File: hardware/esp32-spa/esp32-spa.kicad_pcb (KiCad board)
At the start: 2 copper layers, 17 parts, among them J1 RJ45, J2 RJ45, U1 ESP32-DevKitC-32E, U2 PC817, U3 PC817, U4 PC817, U5 PC817

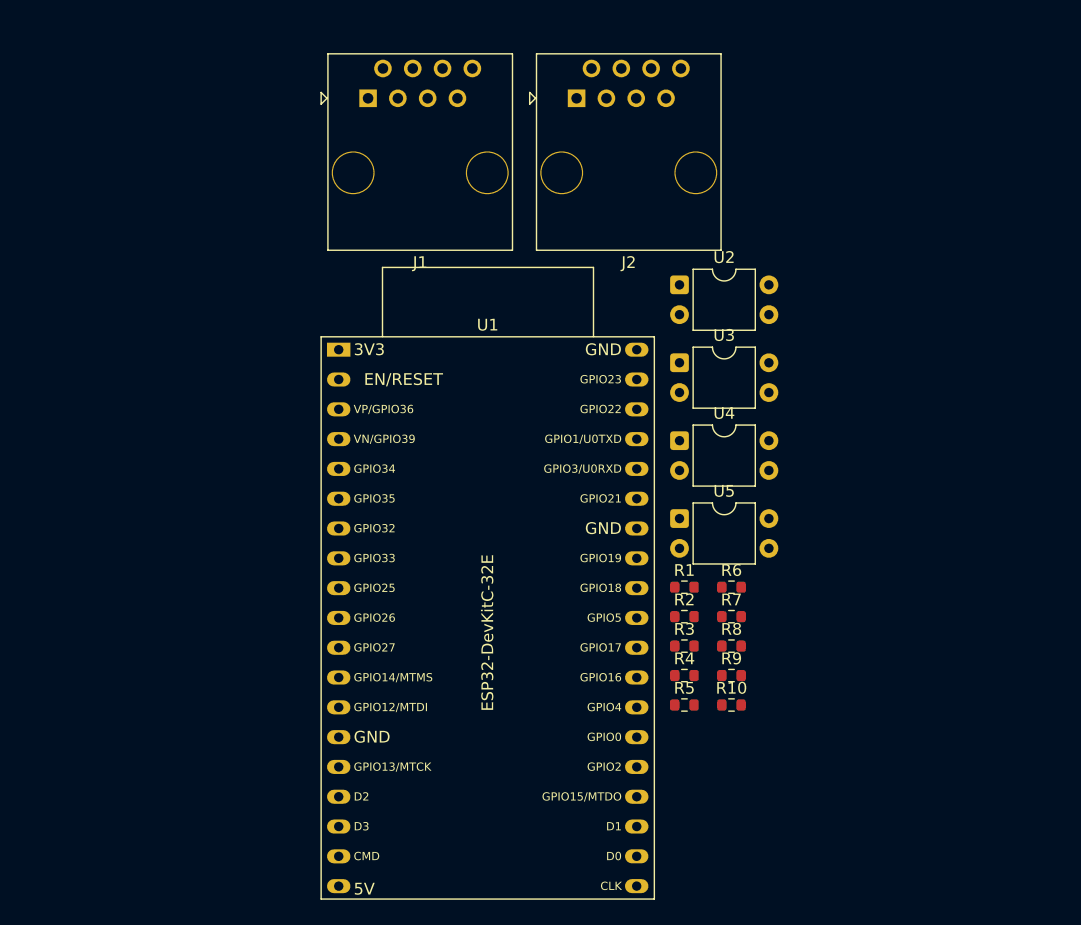
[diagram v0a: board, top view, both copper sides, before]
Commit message: Reorganized pcb layout
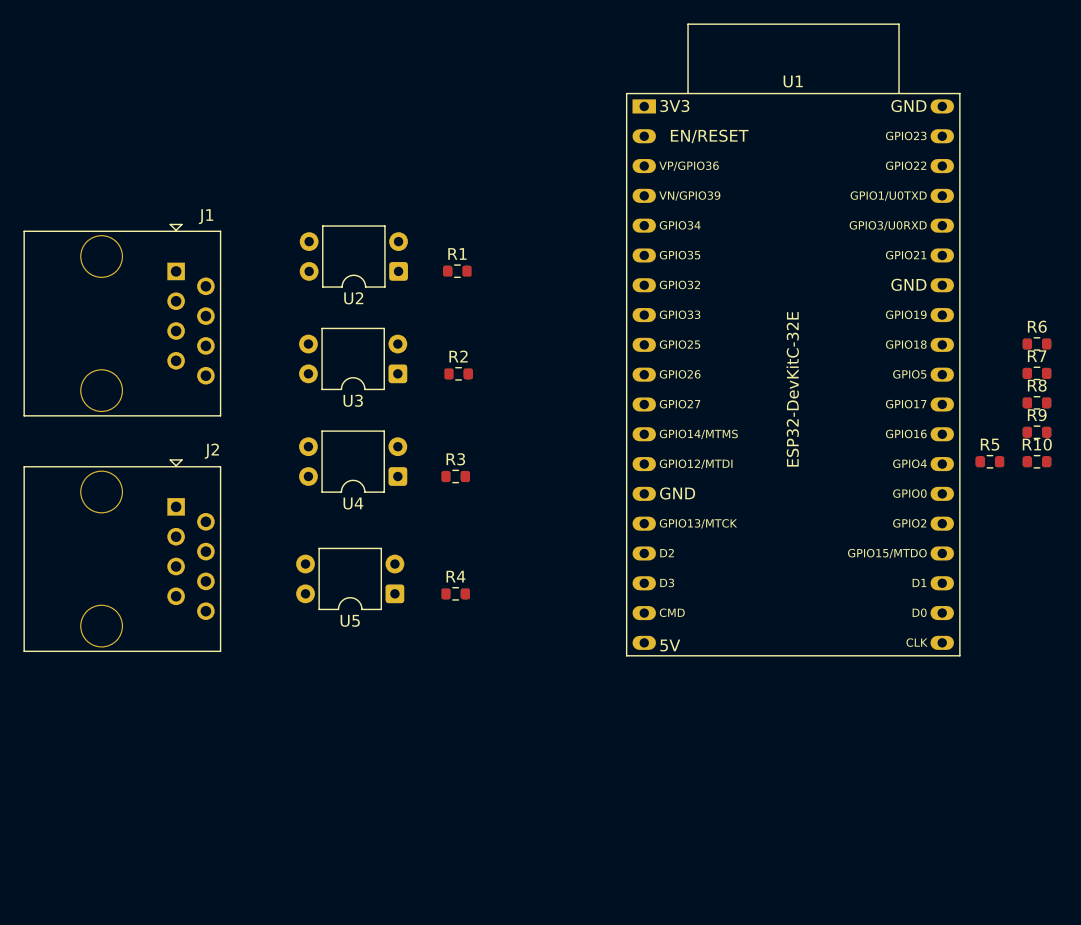
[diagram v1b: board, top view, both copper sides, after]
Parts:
- moved J2 48.8 mm to (123.7, 100.0), turned to -90 degrees
- moved R10 33.3 mm to (197.1, 96.2)
- moved R5 33.3 mm to (193.1, 96.2)
- moved R6 33.3 mm to (197.1, 86.1)
- moved R7 33.3 mm to (197.1, 88.6)
- moved R8 33.3 mm to (197.1, 91.2)
- moved R9 33.3 mm to (197.1, 93.7)
- moved U1 33.3 mm to (163.6, 65.9)
- moved R1 33.2 mm to (147.7, 79.9)
- moved R2 28.3 mm to (147.8, 88.7)
- moved U5 25.1 mm to (142.3, 107.4), turned to 180 degrees
- moved R3 24.3 mm to (147.5, 97.4)
- moved U4 24.2 mm to (142.6, 97.4), turned to 180 degrees
- moved U3 24.0 mm to (142.6, 88.7), turned to 180 degrees
- moved U2 24.0 mm to (142.7, 80.0), turned to 180 degrees
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
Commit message: Remap topside buttons to the measured VL240 pinout
Measured on a new VL240: Warm 7, Cool 3, Light 2, Jets 8 (was 2/8/3/7).
Relabel the optocoupler outputs in the schematic, update the PCB nets and
the README wiring table. Firmware is unchanged; buttons keep their GPIOs.

Also add a logic-analyzer troubleshooting doc for the display tap, which
currently decodes no frames, and update the firmware README status.
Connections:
- U2 pad 3: /RJ45_PIN2 -> /RJ45_PIN7
- U3 pad 3: /RJ45_PIN8 -> /RJ45_PIN3
- U4 pad 3: /RJ45_PIN3 -> /RJ45_PIN2
- U5 pad 3: /RJ45_PIN7 -> /RJ45_PIN8
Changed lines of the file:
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@@
 			(layers "*.Cu" "*.Mask")
 			(remove_unused_layers no)
-			(net "/RJ45_PIN3")
+			(net "/RJ45_PIN2")
 			(pintype "passive")
 		)
@@
 			(layers "*.Cu" "*.Mask")
 			(remove_unused_layers no)
-			(net "/RJ45_PIN8")
+			(net "/RJ45_PIN3")
 			(pintype "passive")
 		)
@@
 			(layers "*.Cu" "*.Mask")
 			(remove_unused_layers no)
-			(net "/RJ45_PIN2")
+			(net "/RJ45_PIN7")
 			(pintype "passive")
 		)
@@
 			(layers "*.Cu" "*.Mask")
 			(remove_unused_layers no)
-			(net "/RJ45_PIN7")
+			(net "/RJ45_PIN8")
 			(pintype "passive")
 		)
